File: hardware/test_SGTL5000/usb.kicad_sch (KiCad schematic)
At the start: 4 parts, among them J401 USB_C_Receptacle_USB2.0, U401 USBLC6-2SC6

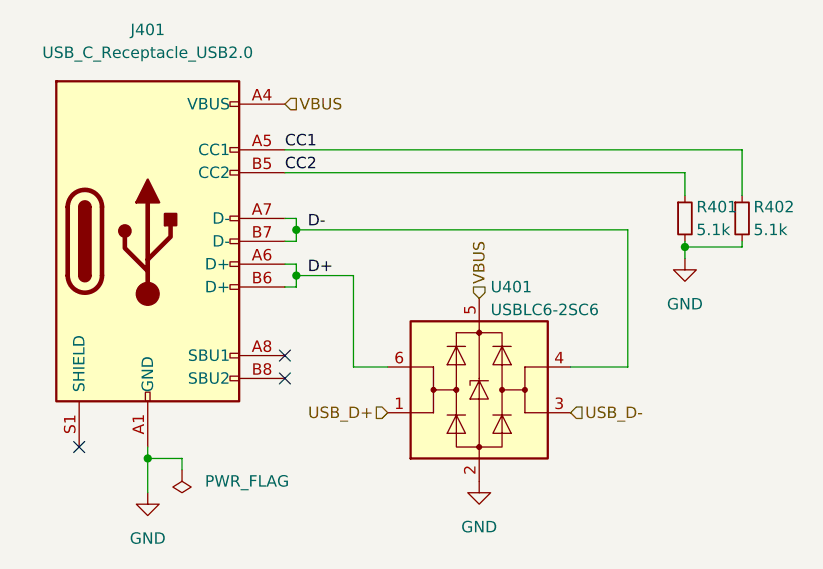
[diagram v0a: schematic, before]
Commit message: routing
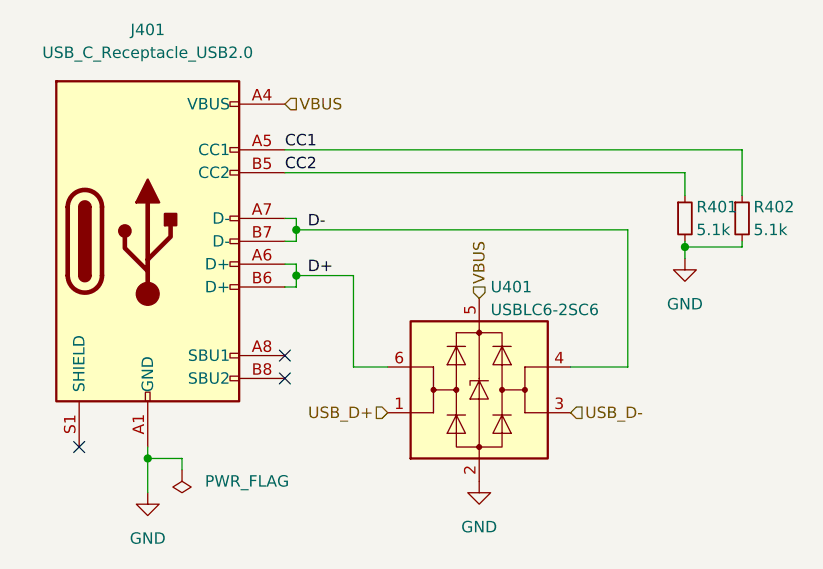
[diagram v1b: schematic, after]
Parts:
- R401, R402: footprint Resistor_SMD:R_0603_1608Metric_Pad0.98x0.95mm_HandSolder -> Resistor_SMD:R_0603_1608Metric
